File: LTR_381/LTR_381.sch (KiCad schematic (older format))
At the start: 21 parts, among them J1 Conn_01x06, J2 Conn_01x04, J3 Conn_01x06, J4 Conn_01x04, Q1 BSS138DW, Q2 BSS138DW, U1 AP2127K-3.3, U2 LTR-381RGB-WA

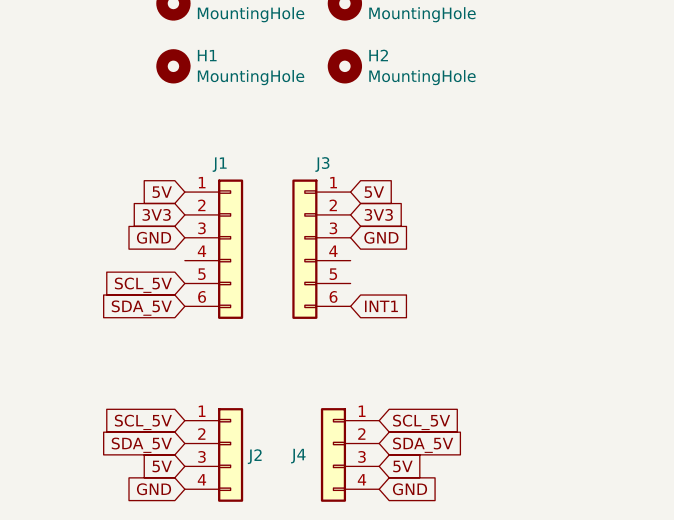
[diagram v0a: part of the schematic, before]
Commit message: Phew...
almost a screw up
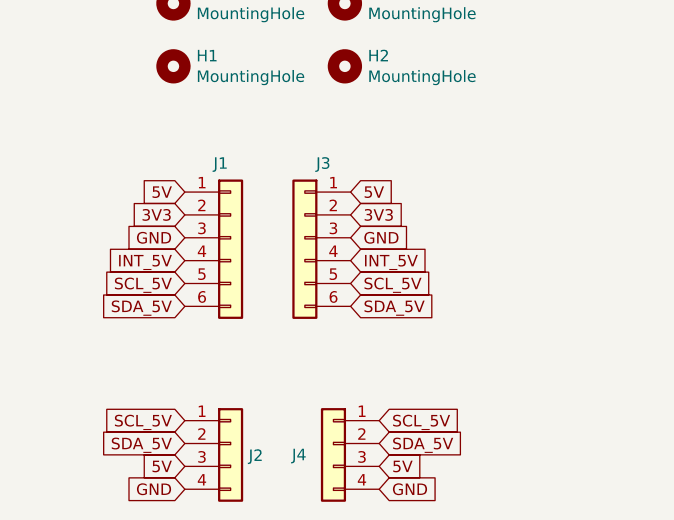
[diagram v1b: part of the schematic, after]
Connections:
- net INT1 is gone; now on net SDA_5V: J3.6 (Pin_6)
- net INT_5V: now also J1.4 (Pin_4), J3.4 (Pin_4)
- net SCL_5V: now also J3.5 (Pin_5)
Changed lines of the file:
@@
 Sheet 1 1
 Title "LTR-381RGB Breakout with 5V Level Shift"
-Date "2020-01-29"
-Rev "1"
+Date "2020-03-10"
+Rev "2"
 Comp "SirBoard"
 Comment1 "Automatic rejection for 50Hz/60Hz lighting"
@@
 	1    0    0    -1
 $EndComp
-Text GLabel 1975 4125 2    50   Input ~ 0
-INT1
+Text GLabel 1975 3925 2    50   Input ~ 0
+INT_5V
 Text GLabel 1250 3825 0    50   Input ~ 0
 GND
@@
 Text GLabel 1975 3825 2    50   Input ~ 0
 GND
+Text GLabel 1250 3925 0    50   Input ~ 0
+INT_5V
+Text GLabel 1975 4025 2    50   Input ~ 0
+SCL_5V
+Text GLabel 1975 4125 2    50   Input ~ 0
+SDA_5V
 $EndSCHEMATC

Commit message: Auto stash before revert of "Board Revision"
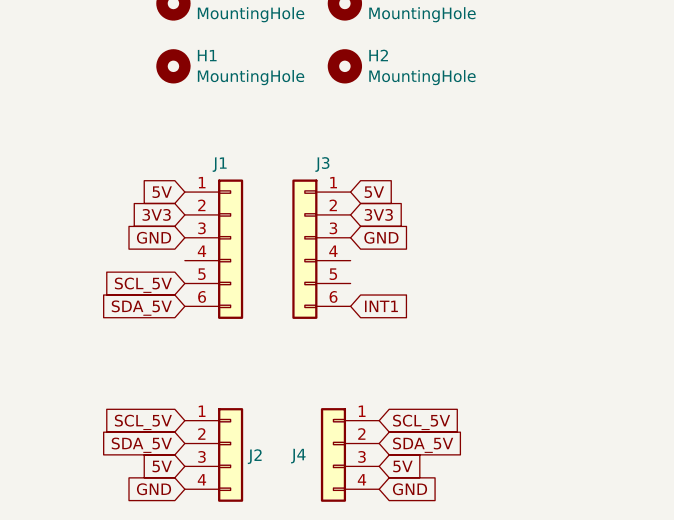
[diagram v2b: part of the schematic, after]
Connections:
- net INT_5V: no longer J1.4 (Pin_4), J3.4 (Pin_4)
- net SCL_5V: no longer J3.5 (Pin_5)
- net SDA_5V: no longer J3.6 (Pin_6)
- new net INT1: J3.6 (Pin_6)
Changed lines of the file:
@@
 Sheet 1 1
 Title "LTR-381RGB Breakout with 5V Level Shift"
-Date "2020-03-10"
-Rev "2"
+Date "2020-01-29"
+Rev "1"
 Comp "SirBoard"
 Comment1 "Automatic rejection for 50Hz/60Hz lighting"
@@
 	1    0    0    -1
 $EndComp
-Text GLabel 1975 3925 2    50   Input ~ 0
-INT_5V
+Text GLabel 1975 4125 2    50   Input ~ 0
+INT1
 Text GLabel 1250 3825 0    50   Input ~ 0
 GND
@@
 Text GLabel 1975 3825 2    50   Input ~ 0
 GND
-Text GLabel 1250 3925 0    50   Input ~ 0
-INT_5V
-Text GLabel 1975 4025 2    50   Input ~ 0
-SCL_5V
-Text GLabel 1975 4125 2    50   Input ~ 0
-SDA_5V
 $EndSCHEMATC
